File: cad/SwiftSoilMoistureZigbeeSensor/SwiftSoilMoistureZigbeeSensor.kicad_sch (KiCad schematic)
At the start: 13 parts, among them J1 Probe, J2 BAT, J3 ARM SWD, Q1 BSS84, SW1 Factory Reset, U1 TPS61221DCK, U2 E73-2G4M08S1C

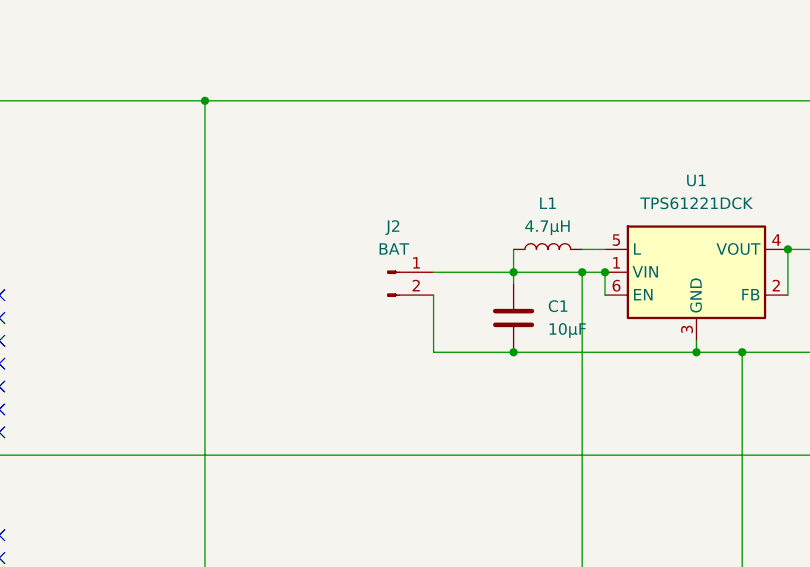
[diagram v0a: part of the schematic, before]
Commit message: PCB Version 1.1
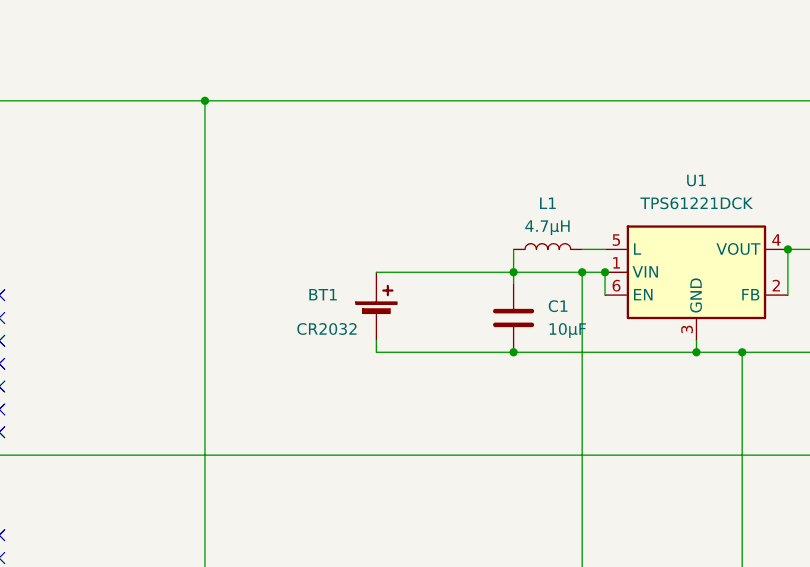
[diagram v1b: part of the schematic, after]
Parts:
- removed J2: BAT, Connector_PinHeader_2.54mm:PinHeader_1x02_P2.54mm_Vertical, symbol Connector:Conn_01x02_Pin
- added BT1: CR2032, Battery:BatteryHolder_Keystone_1060_1x2032, symbol Device:Battery_Cell
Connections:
- net GND: now also BT1.2 (-)
- net at C1.1, L1.1, U1.1 (VIN)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: now also BT1.1 (+)
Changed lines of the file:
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@@
-    (stroke (width 0) (type default))
-  )
-  (wire (pts (xy 162.56 54.61) (xy 162.56 60.96))
     (stroke (width 0) (type default))
   )
@@
     (stroke (width 0) (type default))
   )
-  (wire (pts (xy 162.56 52.07) (xy 171.45 52.07))
+  (wire (pts (xy 156.21 52.07) (xy 171.45 52.07))
     (stroke (width 0) (type default))
   )
@@
     (stroke (width 0) (type default))
   )
-  (wire (pts (xy 162.56 60.96) (xy 171.45 60.96))
+  (wire (pts (xy 156.21 60.96) (xy 171.45 60.96))
+    (stroke (width 0) (type default))
+  )
+  (wire (pts (xy 156.21 60.96) (xy 156.21 59.69))
     (stroke (width 0) (type default))
   )
@@
         (path "/abcc6947-5804-4900-9240-6fa6b27c7542"
           (reference "L1") (unit 1)
-        )
-      )
-    )
-  )
-  (symbol (lib_id "Connector:Conn_01x02_Pin") (at 157.48 52.07 0) (unit 1)
-    (in_bom yes) (on_board yes) (dnp no) (fields_autoplaced)
-    (property "Reference" "J2" (at 158.115 46.99 0)
-      (effects (font (size 1.27 1.27)))
-    )
-    (property "Value" "BAT" (at 158.115 49.53 0)
-      (effects (font (size 1.27 1.27)))
-    )
-    (property "Footprint" "Connector_PinHeader_2.54mm:PinHeader_1x02_P2.54mm_Vertical" (at 157.48 52.07 0)
-      (effects (font (size 1.27 1.27)) hide)
-    )
-    (property "Datasheet" "~" (at 157.48 52.07 0)
-      (effects (font (size 1.27 1.27)) hide)
-    )
-    (property "LCSC" "C180247" (at 157.48 52.07 0)
-      (effects (font (size 1.27 1.27)) hide)
-    )
-    (pin "1")
-    (pin "2")
-    (instances
-      (project "SwiftSoilMoistureZigbeeSensor"
-        (path "/abcc6947-5804-4900-9240-6fa6b27c7542"
-          (reference "J2") (unit 1)
         )
       )
@@
         )
       )
+    )
+  )
+  (symbol (lib_id "Device:Battery_Cell") (at 156.21 57.15 0) (unit 1)
+    (in_bom yes) (on_board yes) (dnp no)
+    (property "Reference" "BT1" (at 148.59 54.61 0)
+      (effects (font (size 1.27 1.27)) (justify left))
+    )
+    (property "Value" "CR2032" (at 147.32 58.42 0)
+      (effects (font (size 1.27 1.27)) (justify left))
+    )
+    (property "Footprint" "Battery:BatteryHolder_Keystone_1060_1x2032" (at 156.21 55.626 90)
+      (effects (font (size 1.27 1.27)) hide)
+    )
+    (property "Datasheet" "~" (at 156.21 55.626 90)
+      (effects (font (size 1.27 1.27)) hide)
+    )
+    (pin "2")
+    (pin "1")
+    (instances
+      (project "SwiftSoilMoistureZigbeeSensor"
+        (path "/abcc6947-5804-4900-9240-6fa6b27c7542"
+          (reference "BT1") (unit 1)
+        )
+      )
